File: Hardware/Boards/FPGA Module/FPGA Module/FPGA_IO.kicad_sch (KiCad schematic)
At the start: 1 part, among them U1 XCKU3P-FFVA676

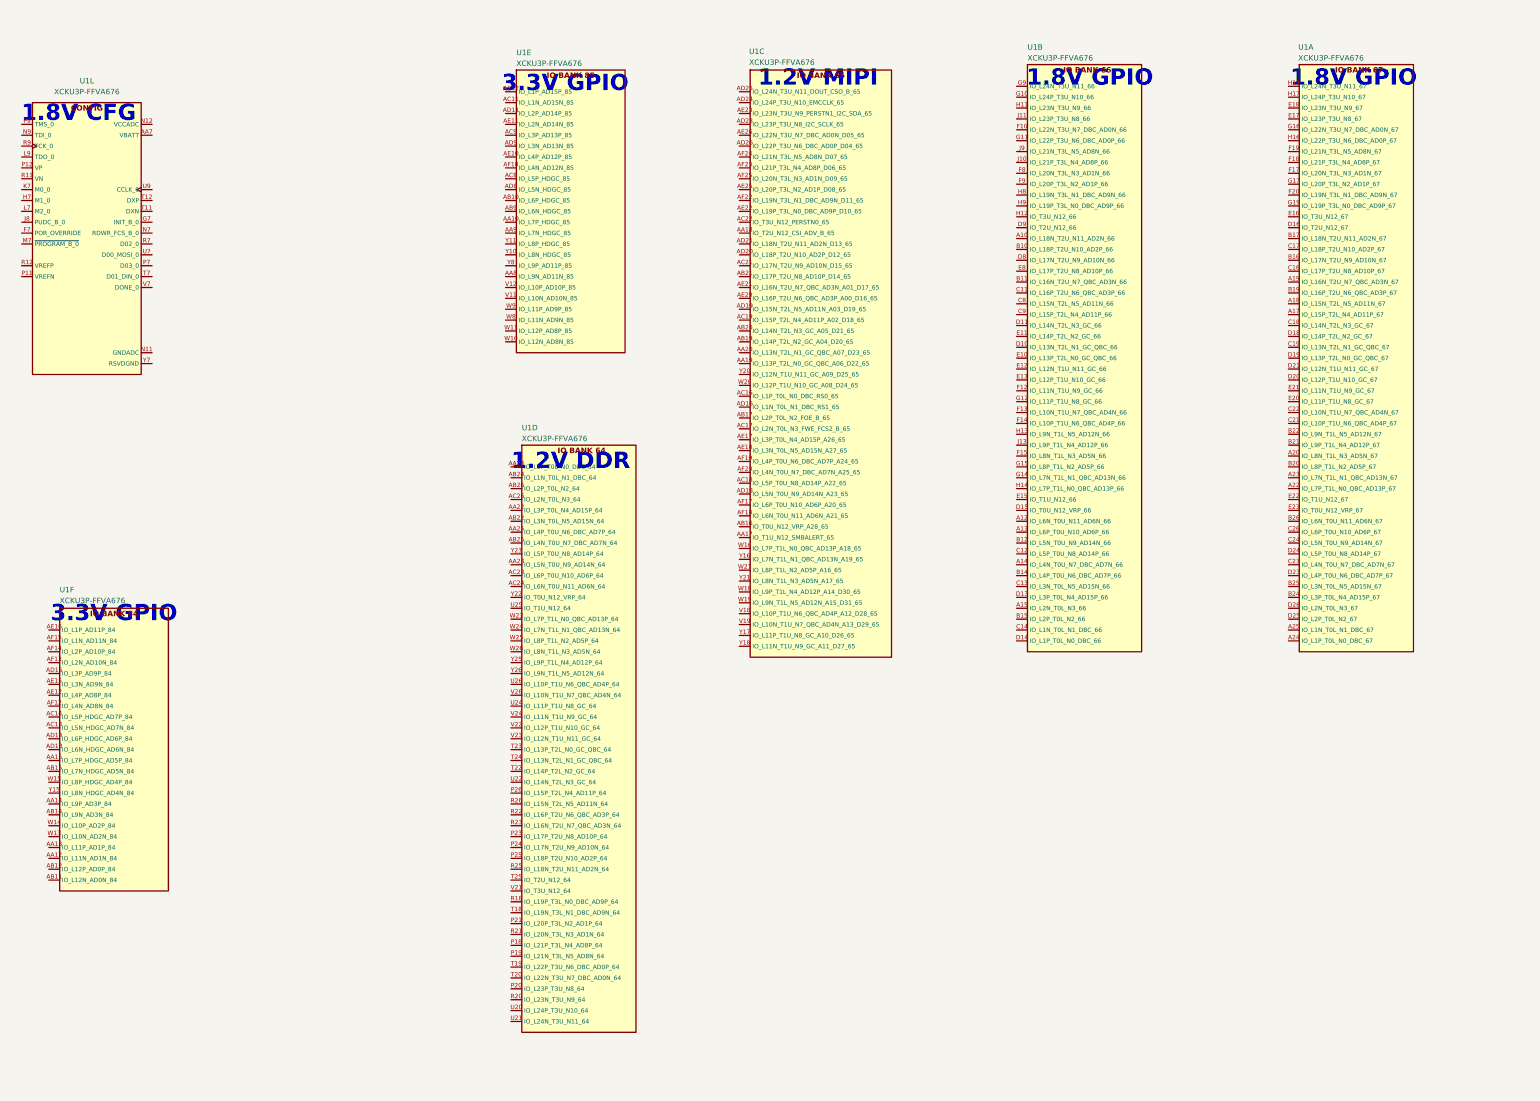
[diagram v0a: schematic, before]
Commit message: Added FPGA Config page
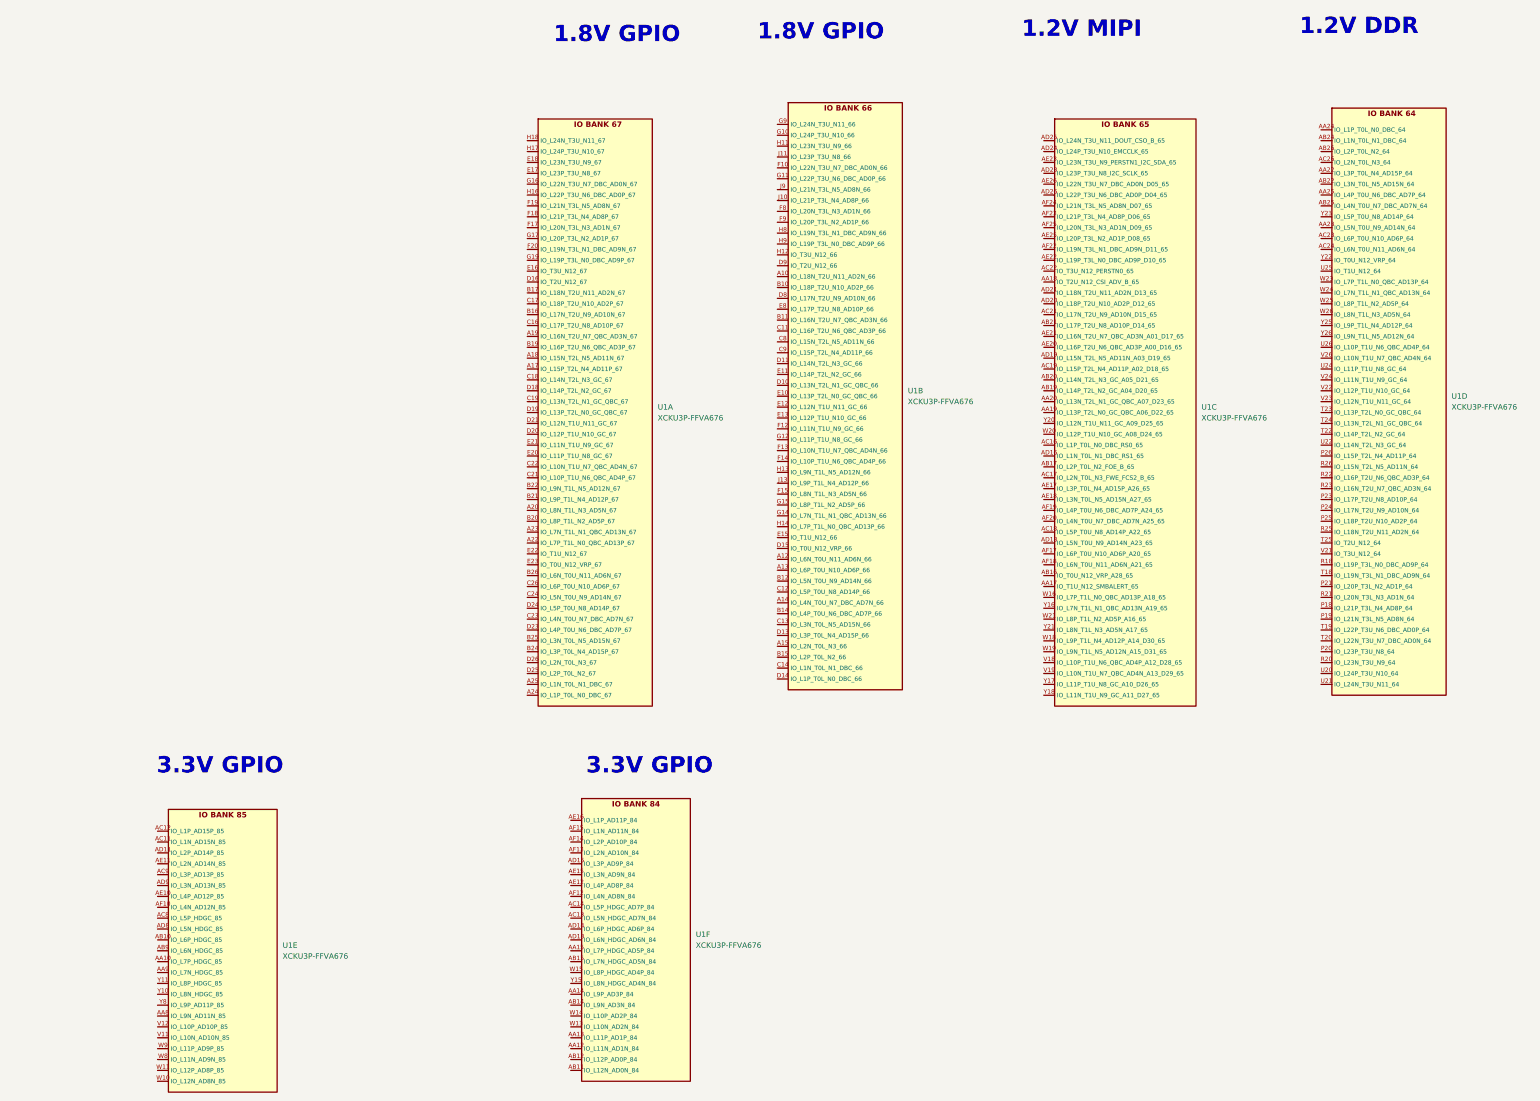
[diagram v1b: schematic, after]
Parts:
- removed U1: XCKU3P-FFVA676, DICE_FPGA_Module:BGA676, symbol DICE_FPGA_Module:XCKU3P-FFVA676
- added U1: XCKU3P-FFVA676, FPGA Module:BGA676, symbol FPGA Module:XCKU3P-FFVA676
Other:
- note removed: "1.8V CFG"
